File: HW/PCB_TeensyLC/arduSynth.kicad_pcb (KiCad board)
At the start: 2 copper layers, 100.3 x 100.3 mm, 36 parts, among them J1 AudioJack3_Ground, J10 Conn_01x03_Male, J11 Screw_Terminal_01x02, J12 Conn_01x02_Male, J13 Conn_01x02_Male, J14 Screw_Terminal_01x02, J2 Conn_01x03_Male, J3 Conn_01x03_Male, J4 Conn_01x03_Male, J5 Conn_01x03_Male, J6 Conn_01x03_Male, J7 Conn_01x03_Male, J8 Conn_01x03_Male, J9 Conn_01x03_Male, SW1 SW_Push, SW2 SW_Push, SW3 SW_Push, SW4 SW_Push, U1 Teensy-LC

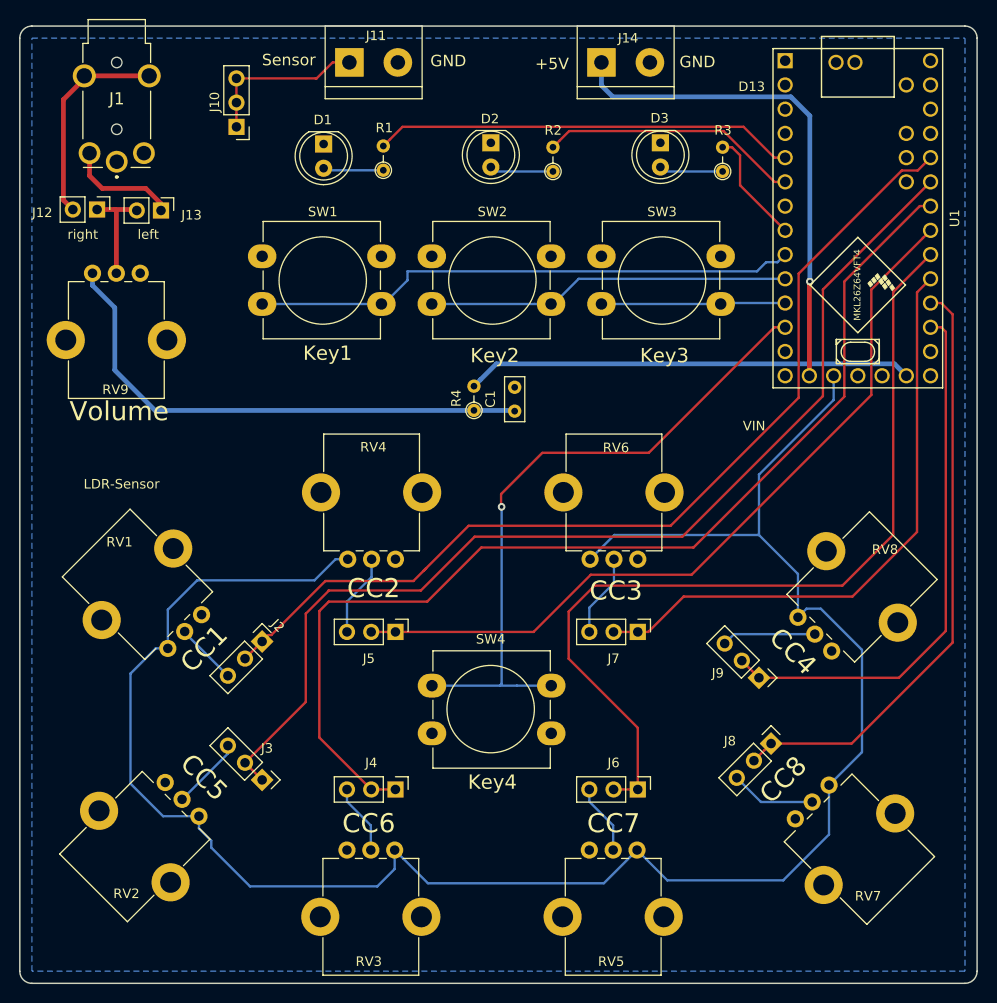
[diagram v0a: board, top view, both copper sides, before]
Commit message: updates for TeensyLC Version
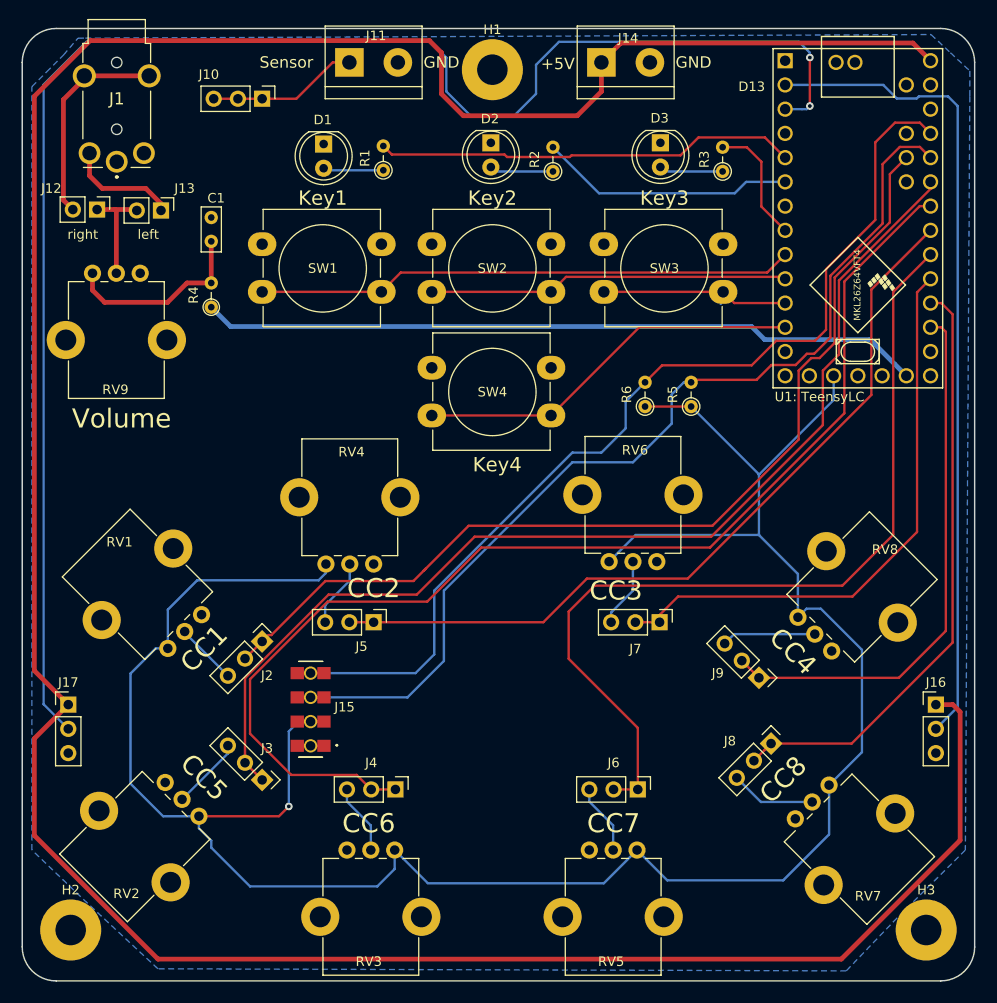
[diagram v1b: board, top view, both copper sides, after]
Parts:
- added H1: MountingHole, MountingHole:MountingHole_3.2mm_M3_Pad, F.Cu at (62.2, 78.2)
- added H2: MountingHole, MountingHole:MountingHole_3.2mm_M3_Pad, F.Cu at (18.0, 168.4)
- added H3: MountingHole, MountingHole:MountingHole_3.2mm_M3_Pad, F.Cu at (107.7, 168.4)
- added J15: display_connector_91601-304LF, TeensySynth_Footprints:91601304LF, F.Cu at (43.2, 145.3)
- added J16: Conn_01x03_Male, Connector_PinHeader_2.54mm:PinHeader_1x03_P2.54mm_Vertical, F.Cu at (108.7, 144.8)
- added J17: Conn_01x03_Male, Connector_PinHeader_2.54mm:PinHeader_1x03_P2.54mm_Vertical, F.Cu at (17.8, 144.8)
- added R5: 4.7K, Resistor_THT:R_Axial_DIN0204_L3.6mm_D1.6mm_P2.54mm_Vertical, F.Cu at (83.1, 113.5)
- added R6: 4.7K, Resistor_THT:R_Axial_DIN0204_L3.6mm_D1.6mm_P2.54mm_Vertical, F.Cu at (78.2, 113.5)
- J1: footprint test:FC68125 -> TeensySynth_Footprints:FC68125
- R1, R2, R3: footprint Resistors_THT:R_Axial_DIN0204_L3.6mm_D1.6mm_P2.54mm_Vertical -> Resistor_THT:R_Axial_DIN0204_L3.6mm_D1.6mm_P2.54mm_Vertical
- U1: TeensyLC: renamed from U1; footprint Teensy:Teensy_LC -> TeensySynth_Footprints:Teensy_LC
- moved SW4 40.3 mm to (55.9, 109.5), turned to 0 degrees
- moved C1 36.4 mm to (32.8, 96.2)
- moved R4 29.6 mm to (32.8, 103.1)
- moved J10 3.99 mm to (38.1, 81.3), turned to 270 degrees
- moved J5 2.50 mm to (49.8, 136.1)
- moved J7 2.50 mm to (79.8, 136.1)
- moved RV4 2.34 mm to (49.8, 130.0)
- moved RV6 2.01 mm to (79.5, 129.8)
- moved SW3 1.30 mm to (73.9, 96.5)
- moved SW1 1.27 mm to (38.1, 96.5)
- moved SW2 1.27 mm to (55.9, 96.5)
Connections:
- R4 pad 1: Net-(C1-Pad1) -> AudioOut
- R4 pad 2: Net-(R4-Pad2) -> Net-(C1-Pad1)
- U1: TeensyLC pad 15: +5V -> Net-(U1-Pad15)
- U1: TeensyLC pad 19: Net-(R4-Pad2) -> AudioOut
- U1: TeensyLC pad 2: Net-(U1-Pad2) -> DataIn
- U1: TeensyLC pad 29: Net-(J2-Pad1) -> SCL
- U1: TeensyLC pad 3: Net-(U1-Pad3) -> DataOut
- U1: TeensyLC pad 30: Net-(U1-Pad30) -> SDA
- U1: TeensyLC pad 33: Net-(U1-Pad33) -> +5V
- U1: TeensyLC pad 36: Net-(U1-Pad36) -> Net-(J2-Pad1)
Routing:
- net +5V: track 52.8 -> 312.1 mm, vias 1 -> 0
- net DataOut: track 0.00 -> 169.8 mm, vias 0 -> 2
- net SDA: track 0.00 -> 106.2 mm
- net SCL: track 0.00 -> 105.7 mm
- net DataIn: track 0.00 -> 85.4 mm
- net AudioOut: track 0.00 -> 75.8 mm
- net Net-(R4-Pad2): track 46.8 -> 0.00 mm
- net Net-(C1-Pad1): track 54.8 -> 19.9 mm
- net +3V3: track 208.1 -> 242.1 mm, vias 0 -> 1
- net Net-(SW4-Pad2): track 69.7 -> 40.9 mm, vias 1 -> 0
- net Net-(J4-Pad1): track 112.2 -> 123.3 mm
- net GND: track 0.00 -> 2.80 mm
- net Net-(J7-Pad1): track 63.3 -> 61.0 mm
- net Net-(J5-Pad1): track 82.5 -> 84.4 mm
- net Net-(J10-Pad1): track 17.7 -> 15.8 mm
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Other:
- board size 100.3 x 100.3 mm -> 99.8 x 99.8 mm
- board text removed: "LDR-Sensor"
- board text removed: "VIN"
